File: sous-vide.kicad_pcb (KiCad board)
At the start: 2 copper layers, 95 x 68 mm, 27 parts, among them J2 Conn_01x02, J3 Conn_01x02, J5 Conn_01x02, Q1 2N3904, SW1 SW_Push_Dual, SW2 SW_Push_Dual, U1 node_mcu1.0, U2 RAC01, U3 G5LE, U4 LCD_Backpack, U5 P090S-04F20BR10K

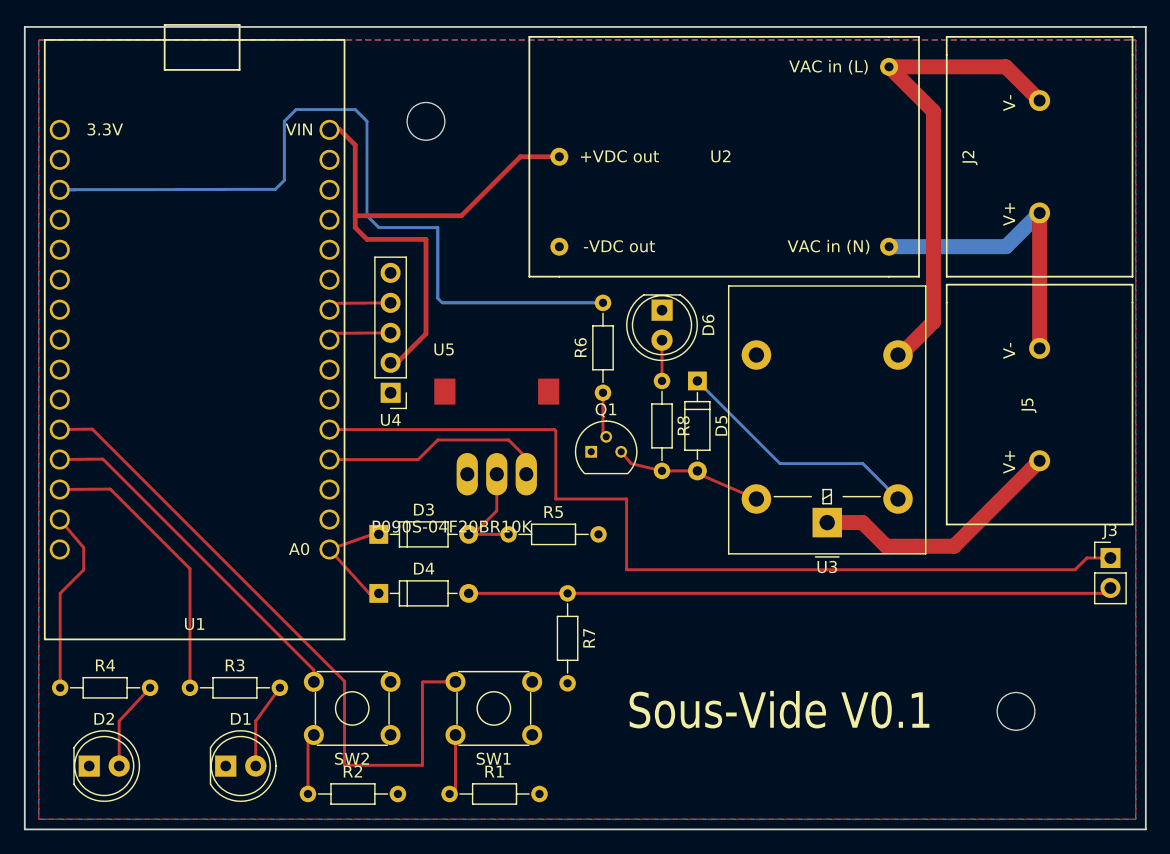
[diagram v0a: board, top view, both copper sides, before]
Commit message: redo entire schematic and layout
now complete with danger zone!
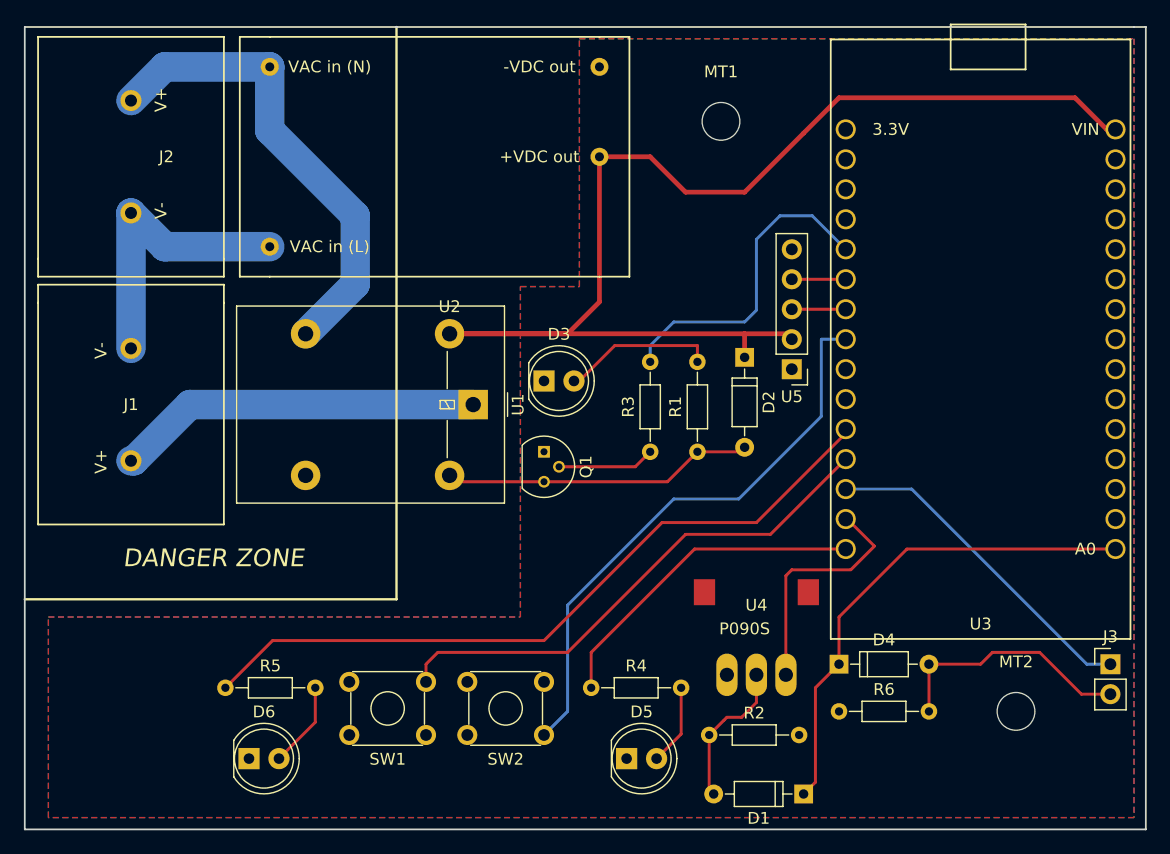
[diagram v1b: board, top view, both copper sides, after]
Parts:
- removed J5: Conn_01x02, custom:NC6-P108-02
- removed R7: 11k, Resistors_THT:R_Axial_DIN0204_L3.6mm_D1.6mm_P7.62mm_Horizontal
- removed R8: 100, Resistors_THT:R_Axial_DIN0204_L3.6mm_D1.6mm_P7.62mm_Horizontal
- removed REF** (x2): MountingHole_3.2mm_M3, Mounting_Holes:MountingHole_3.2mm_M3
- added J1: Conn_01x02, custom:NC6-P108-02, F.Cu at (115.0, 69.0)
- added MT1: MountingHole_3.2mm_M3, Mounting_Holes:MountingHole_3.2mm_M3, F.Cu at (165.0, 45.0)
- added MT2: MountingHole_3.2mm_M3, Mounting_Holes:MountingHole_3.2mm_M3, F.Cu at (190.0, 95.0)
- D1, D2: value LED -> D; footprint LEDs:LED_D5.0mm -> Diodes_THT:D_DO-35_SOD27_P7.62mm_Horizontal
- D3, D5: value D -> LED; footprint Diodes_THT:D_DO-35_SOD27_P7.62mm_Horizontal -> LEDs:LED_D5.0mm
- R1: value 11k -> 110
- R3: value 100 -> 1k
- R4: value 100 -> 41
- R5: value 11k -> 41
- R6: value 1k -> 11k
- U1: value node_mcu1.0 -> G5LE; footprint custom:NodeMCU_1_0 -> Relays_THT:Relay_SPDT_OMRON-G5LE-1
- U3: value G5LE -> node_mcu1.0; footprint Relays_THT:Relay_SPDT_OMRON-G5LE-1 -> custom:NodeMCU_1_0
- U4: value LCD_Backpack -> P090S; footprint Pin_Headers:Pin_Header_Straight_1x05_Pitch2.54mm -> P090S-04F20BR10K:TRIM_P090S-04F20BR10K
- U5: value P090S-04F20BR10K -> LCD_Backpack; footprint P090S-04F20BR10K:TRIM_P090S-04F20BR10K -> Pin_Headers:Pin_Header_Straight_1x05_Pitch2.54mm
- moved J2 77.0 mm to (115.0, 48.0), turned to 90 degrees
- moved D2 65.5 mm to (167.0, 65.0), turned to 270 degrees
- moved D6 51.7 mm to (125.0, 99.0), turned to 0 degrees
- moved D1 49.0 mm to (172.0, 102.0), turned to 180 degrees
- moved R4 45.0 mm to (154.0, 93.0)
- moved R3 43.8 mm to (159.0, 73.0), turned to 90 degrees
- moved D4 39.5 mm to (175.0, 91.0)
- moved U4 35.8 mm to (168.0, 86.0), turned to 0 degrees
- moved R1 35.8 mm to (163.0, 73.0), turned to 90 degrees
- moved R2 34.4 mm to (164.0, 97.0)
- moved R6 33.6 mm to (175.0, 95.0), turned to 0 degrees
- moved D5 32.6 mm to (157.0, 99.0), turned to 0 degrees
- moved R5 27.3 mm to (123.0, 93.0)
- moved U5 25.2 mm to (171.0, 66.0), turned to 180 degrees
- moved U1 23.8 mm to (144.0, 69.0), turned to 270 degrees
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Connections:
- D1 pad 1: GND -> /A0
- D2 pad 1: GND -> +5V
- D3 pad 1: Net-(D3-Pad1) -> GND
- D4 pad 1: Net-(D3-Pad1) -> /A0
- D5 pad 1: Net-(D5-Pad1) -> GND
- J2 pad 2: Net-(J2-Pad2) -> Net-(J1-Pad2)
- J3 pad 1: Net-(J3-Pad1) -> /THERMISTOR
- Q1 pad 3: Net-(D5-Pad2) -> Net-(D2-Pad2)
- R1 pad 1: Net-(R1-Pad1) -> Net-(D2-Pad2)
- R1 pad 2: GND -> Net-(D3-Pad2)
- R2 pad 1: Net-(R2-Pad1) -> Net-(D1-Pad2)
- R3 pad 1: Net-(R3-Pad1) -> Net-(Q1-Pad2)
- R3 pad 2: Net-(D1-Pad2) -> Net-(R3-Pad2)
- R4 pad 1: Net-(R4-Pad1) -> /RED_LED
- R4 pad 2: Net-(D2-Pad2) -> Net-(D5-Pad2)
- R5 pad 1: Net-(D3-Pad2) -> /BLUE_LED
- R5 pad 2: GND -> Net-(D6-Pad2)
- R6 pad 1: Net-(Q1-Pad2) -> GND
- R6 pad 2: Net-(R6-Pad2) -> Net-(D4-Pad2)
- SW1 pad 1: +3V3 -> Net-(SW1-Pad1)
- SW1 pad 2: Net-(R1-Pad1) -> Net-(SW1-Pad2)
- SW1 pad 3: +3V3 -> /SW1
- SW1 pad 4: Net-(SW1-Pad4) -> GND
- SW2 pad 1: +3V3 -> /SW2
- SW2 pad 2: Net-(R2-Pad1) -> GND
- SW2 pad 3: +3V3 -> Net-(SW2-Pad3)
- U1 pad 1: Net-(D3-Pad1) -> Net-(J1-Pad1)
- U1 pad 2: Net-(U1-Pad2) -> +5V
- U1 pad 3: Net-(U1-Pad3) -> Net-(J2-Pad1)
- U1 pad 5: Net-(J3-Pad1) -> Net-(D2-Pad2)
- U2 pad 2: Net-(J2-Pad2) -> Net-(J1-Pad2)
- U3 pad 1: Net-(J5-Pad1) -> /A0
- U3 pad 2: Net-(D5-Pad1) -> (no net)
- U3 pad 3: Net-(J2-Pad2) -> (no net)
- U3 pad 4: Net-(U3-Pad4) -> (no net)
- U3 pad 5: Net-(D5-Pad2) -> (no net)
- U4 pad 2: +5V -> Net-(D1-Pad2)
- U4 pad 3: Net-(U1-Pad8) -> /UESR_POT
- U5 pad 2: Net-(D3-Pad2) -> +5V
- U5 pad 3: Net-(U1-Pad4) -> /CLK
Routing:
- net Net-(J3-Pad1): track 79.2 -> 0.00 mm
- net Net-(R6-Pad2): track 66.7 -> 0.00 mm
- net /BLUE_LED: track 0.00 -> 61.9 mm
- net +5V: track 47.8 -> 106.7 mm
- net Net-(SW1-Pad4): track 56.9 -> 0.00 mm
- net /SW2: track 0.00 -> 48.5 mm
- net /SW1: track 0.00 -> 44.3 mm
- net /A0: track 0.00 -> 42.2 mm
- net Net-(J2-Pad2): track 41.3 -> 0.00 mm
- net Net-(D4-Pad2): track 54.6 -> 21.3 mm
- net Net-(J1-Pad1): track 0.00 -> 31.0 mm
- net Net-(SW2-Pad4): track 29.9 -> 0.00 mm
- net /THERMISTOR: track 0.00 -> 29.6 mm
- net /RED_LED: track 0.00 -> 28.2 mm
- net Net-(R3-Pad2): track 0.00 -> 27.2 mm
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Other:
- net class VAC: clearance 1 -> 2.5; trace_width 1.27 -> 2.5
- board text added: "DANGER ZONE"
- board text removed: "Sous-Vide V0.1"
